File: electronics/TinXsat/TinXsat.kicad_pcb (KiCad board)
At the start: 2 copper layers, 50 x 80 mm, 162 parts, among them J1 USB_B_Mini, J10 CAN, J2 ESP-PROG, J3 POWER_LED, J4 MCO_OUT, J5 BMP280_1, J6 BMP280_2, J7 ESP-card, J8 GPS, J9 SWD, Q1 Si2371, Q2 Si2371, Q3 BSS138, Q4 BSS138, Q5 Si2371, Q6 BSS138, Q7 BSS138, Q8 STD7NK40Z, SW1 SW_Push, U1 CP2102N-A01-GQFN28, U10 TPS61175PWP, U11 STM32F103RGTx, U12 LM35-LP, U13 LM35-LP, U14 LM35-LP, U15 TPS63001, U2 A25L032, U3 MPU-6050, U4 TP4056, U5 Ai-Thinker-Ra-01, U6 ESP32-cam, U7 INA219AxDCN, U8 MCP130, U9 INA219AxDCN, Y1 8Mhz, Y2 32768Hz

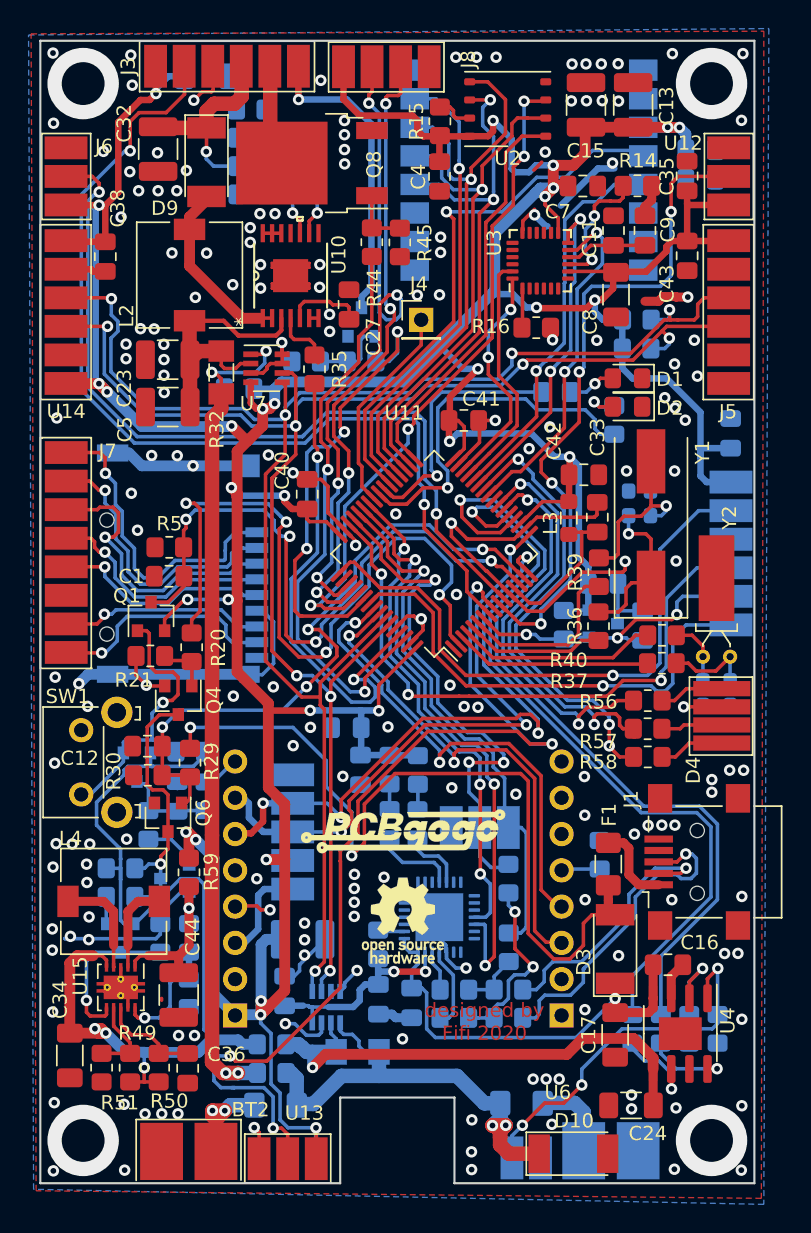
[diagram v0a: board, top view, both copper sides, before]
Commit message: pcb final commit after chinese changes
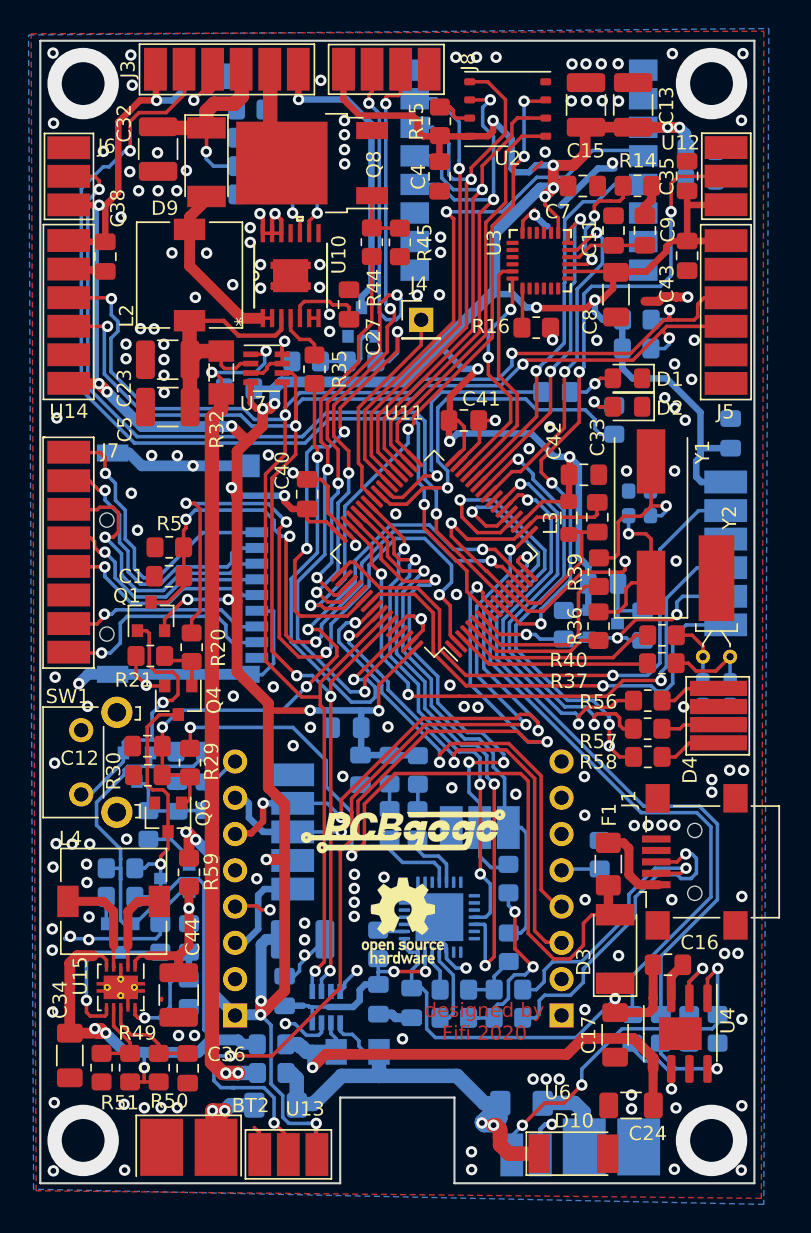
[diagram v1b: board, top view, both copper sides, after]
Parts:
- moved J9 0.37 mm to (98.0, 80.9)
- moved U13 0.30 mm to (69.4, 128.0)
- moved BT2 0.29 mm to (62.3, 127.5)
- moved BT1 0.27 mm to (88.1, 127.5)
- moved D4 0.23 mm to (97.5, 99.2)
- moved TH1 0.21 mm to (83.0, 128.0)
- moved J3 0.21 mm to (58.1, 52.0)
- moved J6 0.19 mm to (52.0, 64.0)
- moved U14 0.19 mm to (52.0, 61.5)
- moved U12 0.18 mm to (98.0, 61.5)
- moved J5 0.18 mm to (98.0, 64.0)
- moved J7 0.18 mm to (52.0, 78.8)
- moved J8 0.17 mm to (71.2, 52.0)
- moved J1 0.17 mm to (95.8, 107.5)
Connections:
- R1 pad 2: +3.3VP -> +3V3
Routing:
- net GND: track 158.6 -> 166.4 mm, vias 180 -> 178
- net BAT_TEMP: track 69.6 -> 66.5 mm
- net Net-(D10-Pad1): track 36.9 -> 34.1 mm
- net +3V3: track 372.1 -> 373.6 mm
- net Net-(J7-Pad1): track 22.1 -> 21.4 mm
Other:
- net class Default: clearance 0.2 -> 0.15
- rule trace_clearance: 0.2 -> 0.15
